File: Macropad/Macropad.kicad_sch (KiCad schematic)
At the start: 63 parts, among them J201 IR_RX, J202 IR_TX, J301 LED_CHAIN, J302 LCD_I2C, J400 BATTERY_LIPO, J401 BAT_PMIC_IO, SW1 SW_Push, SW10 SW_Push, SW11 SW_Push, SW12 SW_Push, SW13 SW_Push, SW14 SW_Push, SW15 SW_Push, SW16 SW_Push, SW17 SW_Push, SW18 SW_Push, SW19 SW_Push, SW2 SW_Push, SW20 SW_Push, SW21 SW_Push, SW22 SW_Push, SW23 SW_Push, SW24 SW_Push, SW25 SW_Push, SW26 SW_Push, SW3 SW_Push, SW4 SW_Push, SW401 RotaryEncoder_Switch, SW5 SW_Push, SW6 SW_Push, SW7 SW_Push, SW8 SW_Push, SW9 SW_Push, U901A ESP32S3_WROOM1_LEFT, U901B ESP32S3_WROOM1_RIGHT

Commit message: Project Updates
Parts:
- J201: value IR_RX -> TSOP4838_C124647
- J202: value IR_TX -> IR333-A_C264290
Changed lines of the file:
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@@
   (symbol
     (lib_id "Connector_Generic:Conn_01x03")
-    (at 290.00 134.00 0)
+    (at 290.00 104.00 0)
     (unit 1)
     (in_bom yes)
     (on_board yes)
     (property "Reference" "J201"
-      (at 290.00 139.00 0)
+      (at 290.00 109.00 0)
       (effects (font (size 1.27 1.27) (thickness 0.15)))
     )
-    (property "Value" "IR_RX"
-      (at 290.00 129.00 0)
+    (property "Value" "TSOP4838_C124647"
+      (at 290.00 99.00 0)
       (effects (font (size 1.27 1.27) (thickness 0.15)))
     )
     (property "Footprint" "Connector_PinHeader_2.54mm:PinHeader_1x03_P2.54mm_Vertical"
-      (at 290.00 134.00 0)
+      (at 290.00 104.00 0)
       (effects (font (size 1.27 1.27) (thickness 0.15)) (hide yes))
     )
     (property "Datasheet" "~"
-      (at 290.00 134.00 0)
+      (at 290.00 104.00 0)
       (effects (font (size 1.27 1.27) (thickness 0.15)) (hide yes))
     )
-    (property "Description" "IR receiver header"
-      (at 290.00 134.00 0)
+    (property "Description" "JLC in-stock IR receiver (TSOP4838, C124647) on SIP-3 footprint"
+      (at 290.00 104.00 0)
       (effects (font (size 1.27 1.27) (thickness 0.15)) (hide yes))
     )
@@
   (symbol
     (lib_id "Connector_Generic:Conn_01x03")
-    (at 290.00 154.00 0)
+    (at 290.00 116.00 0)
     (unit 1)
     (in_bom yes)
     (on_board yes)
     (property "Reference" "J202"
-      (at 290.00 159.00 0)
+      (at 290.00 121.00 0)
       (effects (font (size 1.27 1.27) (thickness 0.15)))
     )
-    (property "Value" "IR_TX"
-      (at 290.00 149.00 0)
+    (property "Value" "IR333-A_C264290"
+      (at 290.00 111.00 0)
       (effects (font (size 1.27 1.27) (thickness 0.15)))
     )
     (property "Footprint" "Connector_PinHeader_2.54mm:PinHeader_1x03_P2.54mm_Vertical"
-      (at 290.00 154.00 0)
+      (at 290.00 116.00 0)
       (effects (font (size 1.27 1.27) (thickness 0.15)) (hide yes))
     )
     (property "Datasheet" "~"
-      (at 290.00 154.00 0)
+      (at 290.00 116.00 0)
       (effects (font (size 1.27 1.27) (thickness 0.15)) (hide yes))
     )
-    (property "Description" "IR transmitter header"
-      (at 290.00 154.00 0)
+    (property "Description" "JLC in-stock IR LED TX (IR333-A, C264290); use driver stage for higher range"
+      (at 290.00 116.00 0)
       (effects (font (size 1.27 1.27) (thickness 0.15)) (hide yes))
     )

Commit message: finished
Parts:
- J302: value LCD_I2C -> LCD_SPI_PWRDATA
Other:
- note added: "LCD: SPI data/clock + power on J302; control (CS/DC/RST/BL) on J303"
- note added: "LED: RGB_DATA (MCU) -> 330R -> LED_DIN, plus 5V/GND (WS2812/SK6812 chain)"
- note removed: "LCD: LCD_SDA/LCD_SCL (I2C) + 3V3/GND on J302"
- note removed: "LED: LED_DATA (MCU) -> 330R -> LED_DIN, plus 5V/GND (WS2812/SK6812 chain)"
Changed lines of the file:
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@@
     (effects (font (size 1.2 1.2) (thickness 0.2)))
   )
-  (text "LED: LED_DATA (MCU) -> 330R -> LED_DIN, plus 5V/GND (WS2812/SK6812 chain)" (at 20.00 42.00 0)
+  (text "LED: RGB_DATA (MCU) -> 330R -> LED_DIN, plus 5V/GND (WS2812/SK6812 chain)" (at 20.00 42.00 0)
     (effects (font (size 1.2 1.2) (thickness 0.2)))
   )
-  (text "LCD: LCD_SDA/LCD_SCL (I2C) + 3V3/GND on J302" (at 20.00 44.50 0)
+  (text "LCD: SPI data/clock + power on J302; control (CS/DC/RST/BL) on J303" (at 20.00 44.50 0)
     (effects (font (size 1.2 1.2) (thickness 0.2)))
   )
@@
       (effects (font (size 1.27 1.27) (thickness 0.15)))
     )
-    (property "Value" "LCD_I2C"
+    (property "Value" "LCD_SPI_PWRDATA"
       (at 332.00 149.00 0)
       (effects (font (size 1.27 1.27) (thickness 0.15)))
@@
     (stroke (width 0) (type default))
   )
-  (global_label "LED_DATA"
+  (global_label "RGB_DATA"
     (shape input)
     (at 322.92 79.08 180)
@@
     (stroke (width 0) (type default))
   )
-  (global_label "LCD_SDA"
+  (global_label "LCD_MOSI"
     (shape input)
     (at 322.92 63.84 180)
@@
     (stroke (width 0) (type default))
   )
-  (global_label "LCD_SCL"
+  (global_label "LCD_SCLK"
     (shape input)
     (at 322.92 61.30 180)
@@
     (stroke (width 0) (type default))
   )
-  (global_label "LCD_SDA"
+  (global_label "LCD_MOSI"
     (shape input)
     (at 322.92 151.46 180)
@@
     (stroke (width 0) (type default))
   )
-  (global_label "LCD_SCL"
+  (global_label "LCD_SCLK"
     (shape input)
     (at 322.92 148.92 180)
@@
     (stroke (width 0) (type default))
   )
-  (global_label "LED_DATA"
+  (global_label "RGB_DATA"
     (shape input)
     (at 301.00 150.00 180)
@@
 			(reference "J302")
 			(unit 1)
-			(value "LCD_I2C")
+			(value "LCD_SPI_PWRDATA")
 			(footprint "Connector_PinHeader_2.54mm:PinHeader_1x04_P2.54mm_Vertical")
 		)

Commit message: DONE DONE DONE
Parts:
- added J303: LCD_SPI_CTRL, Connector_PinHeader_2.54mm:PinHeader_1x04_P2.54mm_Vertical, symbol Connector_Generic:Conn_01x04
- added J304: TOUCH_SD_CTRL, Connector_PinHeader_2.54mm:PinHeader_1x04_P2.54mm_Vertical, symbol Connector_Generic:Conn_01x04
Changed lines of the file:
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@@
+  )
+  (symbol
+    (lib_id "Connector_Generic:Conn_01x04")
+    (at 332.00 166.00 0)
+    (unit 1)
+    (in_bom yes)
+    (on_board yes)
+    (property "Reference" "J303"
+      (at 332.00 171.00 0)
+      (effects (font (size 1.27 1.27) (thickness 0.15)))
+    )
+    (property "Value" "LCD_SPI_CTRL"
+      (at 332.00 161.00 0)
+      (effects (font (size 1.27 1.27) (thickness 0.15)))
+    )
+    (property "Footprint" "Connector_PinHeader_2.54mm:PinHeader_1x04_P2.54mm_Vertical"
+      (at 332.00 166.00 0)
+      (effects (font (size 1.27 1.27) (thickness 0.15)) (hide yes))
+    )
+    (property "Datasheet" "~"
+      (at 332.00 166.00 0)
+      (effects (font (size 1.27 1.27) (thickness 0.15)) (hide yes))
+    )
+    (property "Description" "LCD SPI control header (CS/DC/RST/BL)"
+      (at 332.00 166.00 0)
+      (effects (font (size 1.27 1.27) (thickness 0.15)) (hide yes))
+    )
+    (pin "1")
+    (pin "2")
+    (pin "3")
+    (pin "4")
+  )
+  (symbol
+    (lib_id "Connector_Generic:Conn_01x04")
+    (at 332.00 178.00 0)
+    (unit 1)
+    (in_bom yes)
+    (on_board yes)
+    (property "Reference" "J304"
+      (at 332.00 183.00 0)
+      (effects (font (size 1.27 1.27) (thickness 0.15)))
+    )
+    (property "Value" "TOUCH_SD_CTRL"
+      (at 332.00 173.00 0)
+      (effects (font (size 1.27 1.27) (thickness 0.15)))
+    )
+    (property "Footprint" "Connector_PinHeader_2.54mm:PinHeader_1x04_P2.54mm_Vertical"
+      (at 332.00 178.00 0)
+      (effects (font (size 1.27 1.27) (thickness 0.15)) (hide yes))
+    )
+    (property "Datasheet" "~"
+      (at 332.00 178.00 0)
+      (effects (font (size 1.27 1.27) (thickness 0.15)) (hide yes))
+    )
+    (property "Description" "Touch + SD shared-SPI control header (CS/MISO/IRQ/SD_CS)"
+      (at 332.00 178.00 0)
+      (effects (font (size 1.27 1.27) (thickness 0.15)) (hide yes))
+    )
+    (pin "1")
+    (pin "2")
+    (pin "3")
+    (pin "4")
   )
   (symbol
@@
   )
   (wire
+    (pts (xy 326.92 168.54) (xy 322.92 168.54))
+    (stroke (width 0) (type default))
+  )
+  (global_label "LCD_CS"
+    (shape input)
+    (at 322.92 168.54 180)
+    (fields_autoplaced)
+    (effects (font (size 1.27 1.27) (thickness 0.15)))
+  )
+  (wire
+    (pts (xy 326.92 166.00) (xy 322.92 166.00))
+    (stroke (width 0) (type default))
+  )
+  (global_label "LCD_DC"
+    (shape input)
+    (at 322.92 166.00 180)
+    (fields_autoplaced)
+    (effects (font (size 1.27 1.27) (thickness 0.15)))
+  )
+  (wire
+    (pts (xy 326.92 163.46) (xy 322.92 163.46))
+    (stroke (width 0) (type default))
+  )
+  (global_label "LCD_RST"
+    (shape input)
+    (at 322.92 163.46 180)
+    (fields_autoplaced)
+    (effects (font (size 1.27 1.27) (thickness 0.15)))
+  )
+  (wire
+    (pts (xy 326.92 160.92) (xy 322.92 160.92))
+    (stroke (width 0) (type default))
+  )
+  (global_label "LCD_BL"
+    (shape input)
+    (at 322.92 160.92 180)
+    (fields_autoplaced)
+    (effects (font (size 1.27 1.27) (thickness 0.15)))
+  )
+  (wire
+    (pts (xy 326.92 180.54) (xy 322.92 180.54))
+    (stroke (width 0) (type default))
+  )
+  (global_label "TOUCH_CS"
+    (shape input)
+    (at 322.92 180.54 180)
+    (fields_autoplaced)
+    (effects (font (size 1.27 1.27) (thickness 0.15)))
+  )
+  (wire
+    (pts (xy 326.92 178.00) (xy 322.92 178.00))
+    (stroke (width 0) (type default))
+  )
+  (global_label "TOUCH_MISO"
+    (shape input)
+    (at 322.92 178.00 180)
+    (fields_autoplaced)
+    (effects (font (size 1.27 1.27) (thickness 0.15)))
+  )
+  (wire
+    (pts (xy 326.92 175.46) (xy 322.92 175.46))
+    (stroke (width 0) (type default))
+  )
+  (global_label "TOUCH_IRQ"
+    (shape input)
+    (at 322.92 175.46 180)
+    (fields_autoplaced)
+    (effects (font (size 1.27 1.27) (thickness 0.15)))
+  )
+  (wire
+    (pts (xy 326.92 172.92) (xy 322.92 172.92))
+    (stroke (width 0) (type default))
+  )
+  (global_label "SD_CS"
+    (shape input)
+    (at 322.92 172.92 180)
+    (fields_autoplaced)
+    (effects (font (size 1.27 1.27) (thickness 0.15)))
+  )
+  (wire
     (pts (xy 326.92 135.27) (xy 322.92 135.27))
     (stroke (width 0) (type default))
@@
 			(footprint "Connector_PinHeader_2.54mm:PinHeader_1x04_P2.54mm_Vertical")
 		)
+		(path "/d443aa2d-d6e1-4495-ad62-9712672694e4"
+			(reference "J303")
+			(unit 1)
+			(value "LCD_SPI_CTRL")
+			(footprint "Connector_PinHeader_2.54mm:PinHeader_1x04_P2.54mm_Vertical")
+		)
+		(path "/aabc9772-6793-4e06-a3fe-930a60627d16"
+			(reference "J304")
+			(unit 1)
+			(value "TOUCH_SD_CTRL")
+			(footprint "Connector_PinHeader_2.54mm:PinHeader_1x04_P2.54mm_Vertical")
+		)

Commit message: DONE NOW
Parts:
- J304: value TOUCH_SD_CTRL -> TOUCH_I2C_SD
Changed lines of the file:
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@@
       (effects (font (size 1.27 1.27) (thickness 0.15)))
     )
-    (property "Value" "TOUCH_SD_CTRL"
+    (property "Value" "TOUCH_I2C_SD"
       (at 332.00 173.00 0)
       (effects (font (size 1.27 1.27) (thickness 0.15)))
@@
       (effects (font (size 1.27 1.27) (thickness 0.15)) (hide yes))
     )
-    (property "Description" "Touch + SD shared-SPI control header (CS/MISO/IRQ/SD_CS)"
+    (property "Description" "Touch I2C + SD SPI header (TOUCH_SDA/SPI_MISO/TOUCH_SCL/SD_CS)"
       (at 332.00 178.00 0)
       (effects (font (size 1.27 1.27) (thickness 0.15)) (hide yes))
@@
     (stroke (width 0) (type default))
   )
-  (global_label "TOUCH_CS"
+  (global_label "TOUCH_SDA"
     (shape input)
     (at 322.92 180.54 180)
@@
     (stroke (width 0) (type default))
   )
-  (global_label "TOUCH_MISO"
+  (global_label "SPI_MISO"
     (shape input)
     (at 322.92 178.00 180)
@@
     (stroke (width 0) (type default))
   )
-  (global_label "TOUCH_IRQ"
+  (global_label "TOUCH_SCL"
     (shape input)
     (at 322.92 175.46 180)
@@
 			(reference "J304")
 			(unit 1)
-			(value "TOUCH_SD_CTRL")
+			(value "TOUCH_I2C_SD")
 			(footprint "Connector_PinHeader_2.54mm:PinHeader_1x04_P2.54mm_Vertical")
 		)

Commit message: IR INCREASE
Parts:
- added R408: 220R, Resistor_SMD:R_0603_1608Metric, symbol Device:R
- J202: value IR333-A_C264290 -> IR_LED_TX_HDR
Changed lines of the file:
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@@
       (effects (font (size 1.27 1.27) (thickness 0.15)))
     )
-    (property "Value" "IR333-A_C264290"
+    (property "Value" "IR_LED_TX_HDR"
       (at 290.00 111.00 0)
       (effects (font (size 1.27 1.27) (thickness 0.15)))
@@
       (effects (font (size 1.27 1.27) (thickness 0.15)) (hide yes))
     )
-    (property "Description" "JLC in-stock IR LED TX (IR333-A, C264290); use driver stage for higher range"
+    (property "Description" "IR TX header for bare LED with on-board series current limiting"
       (at 290.00 116.00 0)
       (effects (font (size 1.27 1.27) (thickness 0.15)) (hide yes))
@@
   )
   (symbol
+    (lib_id "Device:R")
+    (at 292.00 146.00 0)
+    (unit 1)
+    (in_bom yes)
+    (on_board yes)
+    (property "Reference" "R408"
+      (at 292.00 149.00 0)
+      (effects (font (size 1.27 1.27) (thickness 0.15)))
+    )
+    (property "Value" "220R"
+      (at 292.00 143.00 0)
+      (effects (font (size 1.27 1.27) (thickness 0.15)))
+    )
+    (property "Footprint" "Resistor_SMD:R_0603_1608Metric"
+      (at 292.00 146.00 0)
+      (effects (font (size 1.27 1.27) (thickness 0.15)) (hide yes))
+    )
+    (property "Datasheet" "~"
+      (at 292.00 146.00 0)
+      (effects (font (size 1.27 1.27) (thickness 0.15)) (hide yes))
+    )
+    (property "Description" "Series current limit for IR TX LED header"
+      (at 292.00 146.00 0)
+      (effects (font (size 1.27 1.27) (thickness 0.15)) (hide yes))
+    )
+    (pin "1")
+    (pin "2")
+  )
+  (symbol
     (lib_id "Device:CP")
     (at 352.00 150.00 0)
@@
     (stroke (width 0) (type default))
   )
+  (global_label "IR_TX_LED"
+    (shape input)
+    (at 280.92 150.19 180)
+    (fields_autoplaced)
+    (effects (font (size 1.27 1.27) (thickness 0.15)))
+  )
+  (wire
+    (pts (xy 289.46 146.00) (xy 286.92 146.00))
+    (stroke (width 0) (type default))
+  )
   (global_label "IR_TX"
     (shape input)
-    (at 280.92 150.19 180)
+    (at 286.92 146.00 180)
+    (fields_autoplaced)
+    (effects (font (size 1.27 1.27) (thickness 0.15)))
+  )
+  (wire
+    (pts (xy 294.54 146.00) (xy 299.08 146.00))
+    (stroke (width 0) (type default))
+  )
+  (global_label "IR_TX_LED"
+    (shape input)
+    (at 299.08 146.00 0)
     (fields_autoplaced)
     (effects (font (size 1.27 1.27) (thickness 0.15)))
@@
 			(footprint "Connector_PinHeader_2.54mm:PinHeader_1x03_P2.54mm_Vertical")
 		)
-		(path "/acbcb9e5-54ca-403f-af24-2c20118682d5"
-			(reference "J202")
-			(unit 1)
-			(value "IR_TX")
-			(footprint "Connector_PinHeader_2.54mm:PinHeader_1x03_P2.54mm_Vertical")
-		)
+			(path "/acbcb9e5-54ca-403f-af24-2c20118682d5"
+				(reference "J202")
+				(unit 1)
+				(value "IR_LED_TX_HDR")
+				(footprint "Connector_PinHeader_2.54mm:PinHeader_1x03_P2.54mm_Vertical")
+			)
+			(path "/c1c331ff-3c3a-4f60-88c7-c036e28a1302"
+				(reference "R408")
+				(unit 1)
+				(value "220R")
+				(footprint "Resistor_SMD:R_0603_1608Metric")
+			)
 		(path "/404ff6c7-148c-438c-a9f2-f16d9f51ed43"
 			(reference "J301")

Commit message: Finalize macropad firmware + schematic/pcb validation updates
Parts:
- C401: symbol Device:CP -> Device:R
- J304: value TOUCH_I2C_SD -> TOUCH_I2C_SD_IRQ; footprint Connector_PinHeader_2.54mm:PinHeader_1x04_P2.54mm_Vertical -> Connector_PinHeader_2.54mm:PinHeader_1x05_P2.54mm_Vertical; symbol Connector_Generic:Conn_01x04 -> Connector_Generic:Conn_01x05
- SW1, SW10, SW11, SW12, SW13, SW14, SW15, SW16, SW17, SW18, SW19, SW2, SW20, SW21, SW22, SW23, SW24, SW25, SW26, SW3, SW4, SW5, SW6, SW7, SW8, SW9: footprint Keyboard:SW_Hotswap_Kailh_MX -> Button_Switch_Keyboard:SW_Cherry_MX_1.00u_PCB
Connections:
- net 3V3: now also J302.3 (Pin_3), U901A.10 (Pin_10)
- net BAT+: now also J401.3 (Pin_3)
- net COL0: now also D1.2 (A), D12.2 (A), D17.2 (A), D2.2 (A), D22.2 (A), D7.2 (A), SW13.1, SW18.1, SW23.1, SW3.1, SW8.1, U901A.3 (Pin_3)
- net COL4: now also D11.2 (A), D16.2 (A), D21.2 (A), D26.2 (A), U901B.9 (Pin_9)
- net ENC_A: now also SW401.B, U901B.5 (Pin_5)
- net ENC_B: now also SW401.A, U901B.4 (Pin_4)
- net ENC_SW: now also SW401.S2, U901B.3 (Pin_3)
- net GND: now also J302.2 (Pin_2), J401.2 (Pin_2), SW401.C, SW401.S1, U901A.11 (Pin_11), U901B.11 (Pin_11)
- net LCD_MOSI: now also J302.1 (Pin_1), U901B.2 (Pin_2)
- net ROW0: now also SW1.1, U901A.9 (Pin_9)
- new net 5V_SYS: J401.1 (Pin_1), U901B.10 (Pin_10)
- new net COL1: D23.2 (A), SW24.1, U901A.2 (Pin_2)
- new net COL2: D24.2 (A), SW25.1, U901A.1 (Pin_1)
- new net COL3: D25.2 (A), SW26.1
- new net ROW1: D4.2 (A), D5.2 (A), SW5.1, SW6.1, U901A.8 (Pin_8)
- new net ROW2: D10.2 (A), SW11.1, U901A.7 (Pin_7)
- new net ROW3: D15.2 (A), SW16.1, U901A.6 (Pin_6)
- new net ROW4: D20.2 (A), SW21.1, U901A.5 (Pin_5)
- no-connect marks 0 -> 113

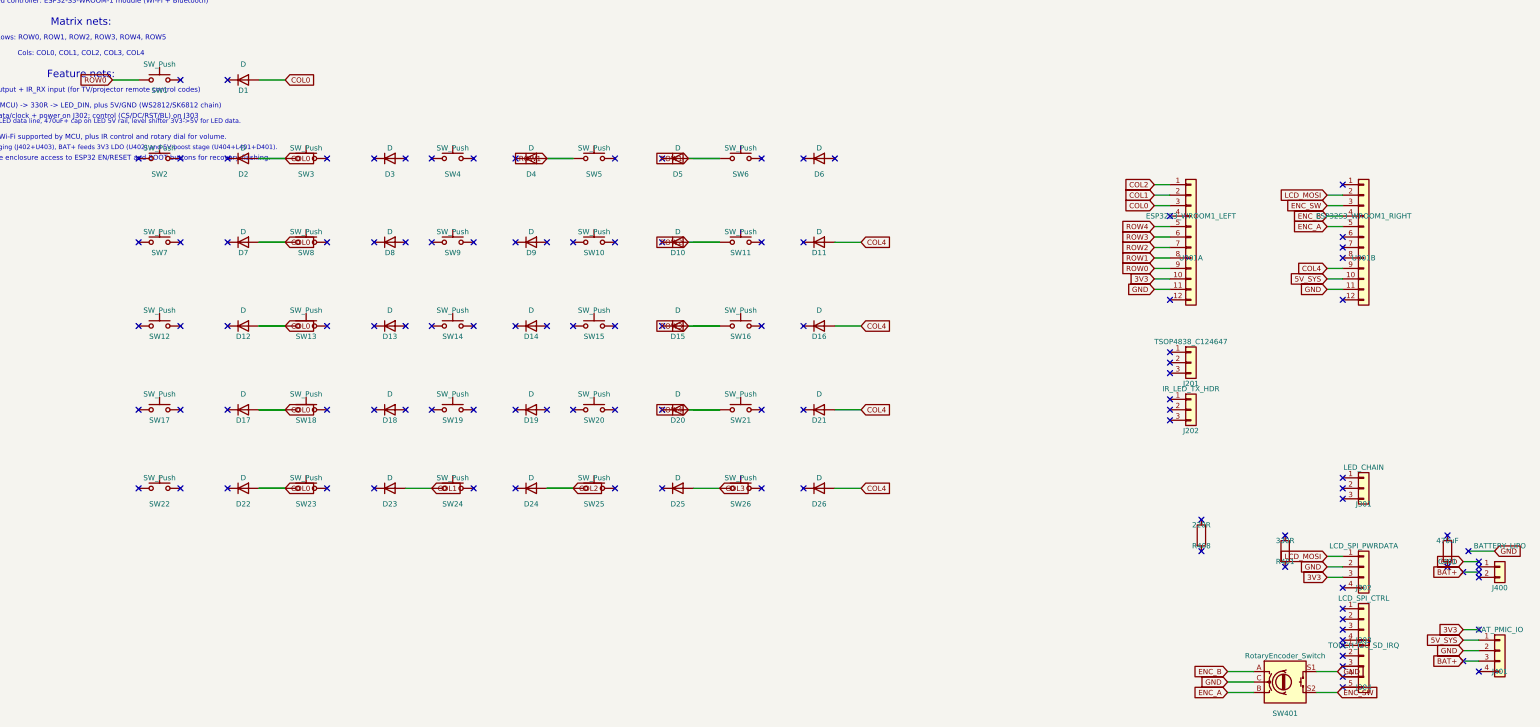
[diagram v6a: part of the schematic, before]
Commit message: FINISHED
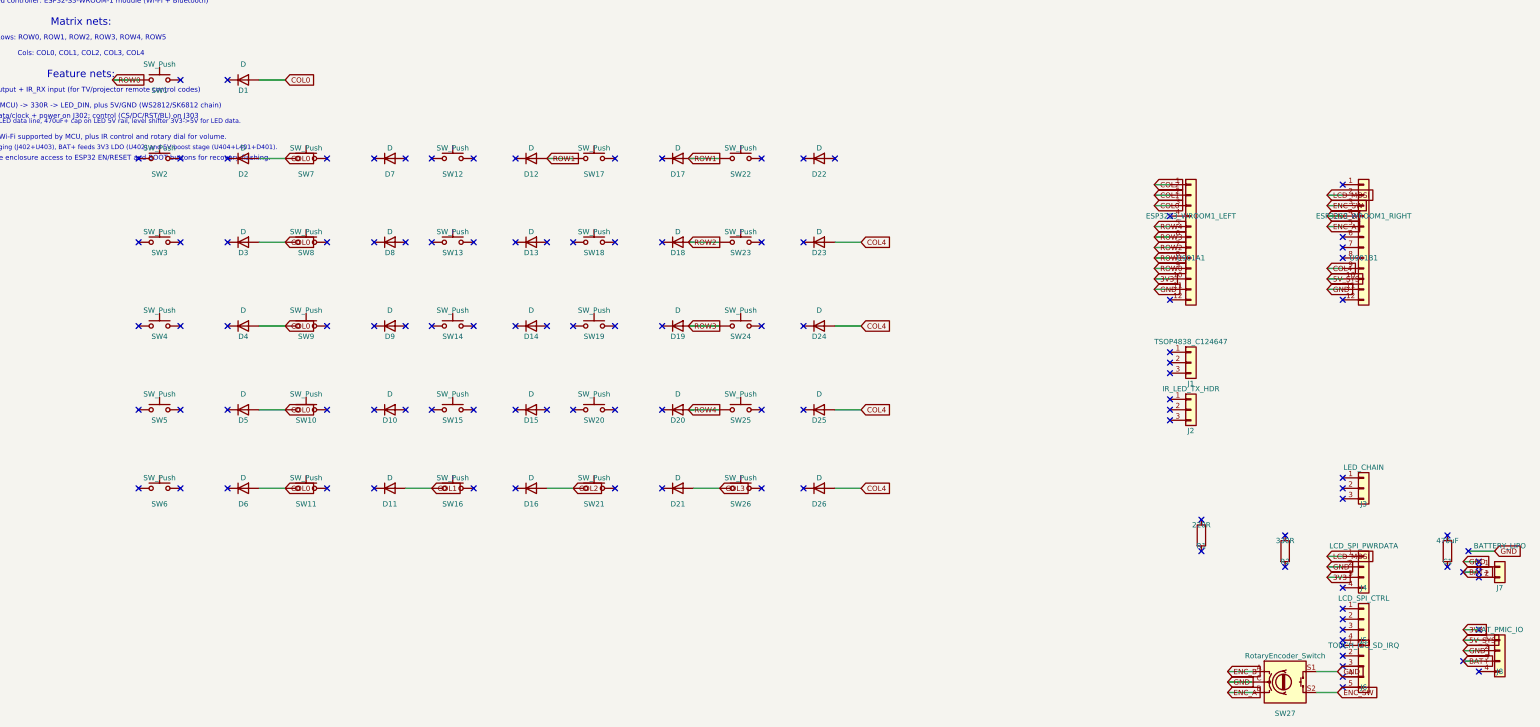
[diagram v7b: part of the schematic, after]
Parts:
- renumbered C401 to C1, D18 to D10, D23 to D11, D4 to D12, D9 to D13, D19 to D15, D24 to D16, D5 to D17, D10 to D18, D15 to D19, D25 to D21, D6 to D22, D11 to D23, D16 to D24, D21 to D25, D7 to D3, D12 to D4, D17 to D5, D22 to D6, D3 to D7, D13 to D9, J201 to J1, J202 to J2, J301 to J3, J302 to J4, J303 to J5, J304 to J6, J400 to J7, J401 to J8, R408 to R1, R401 to R2, SW18 to SW10, SW23 to SW11, SW4 to SW12, SW9 to SW13, SW19 to SW15, SW24 to SW16, SW5 to SW17, SW10 to SW18, SW15 to SW19, SW25 to SW21, SW6 to SW22, SW11 to SW23, SW16 to SW24, SW21 to SW25, SW401 to SW27, SW7 to SW3, SW12 to SW4, SW17 to SW5, SW22 to SW6, SW3 to SW7, SW13 to SW9, U901A to U901A1, U901B to U901B1
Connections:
- net ROW1: no longer D17.2 (A)
- net ROW2: no longer D18.2 (A)
- net ROW3: no longer D19.2 (A)
- net ROW4: no longer D20.2 (A)
